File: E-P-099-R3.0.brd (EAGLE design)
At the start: 113.1 x 96.5 mm, 107 parts, among them J1 AVR_ISP, J2 1445055-3, Q1 BSS101, Q2 BSS101, Q3 BSS101, Q4 BSS101, Q5 BSS101, Q6 BSS101

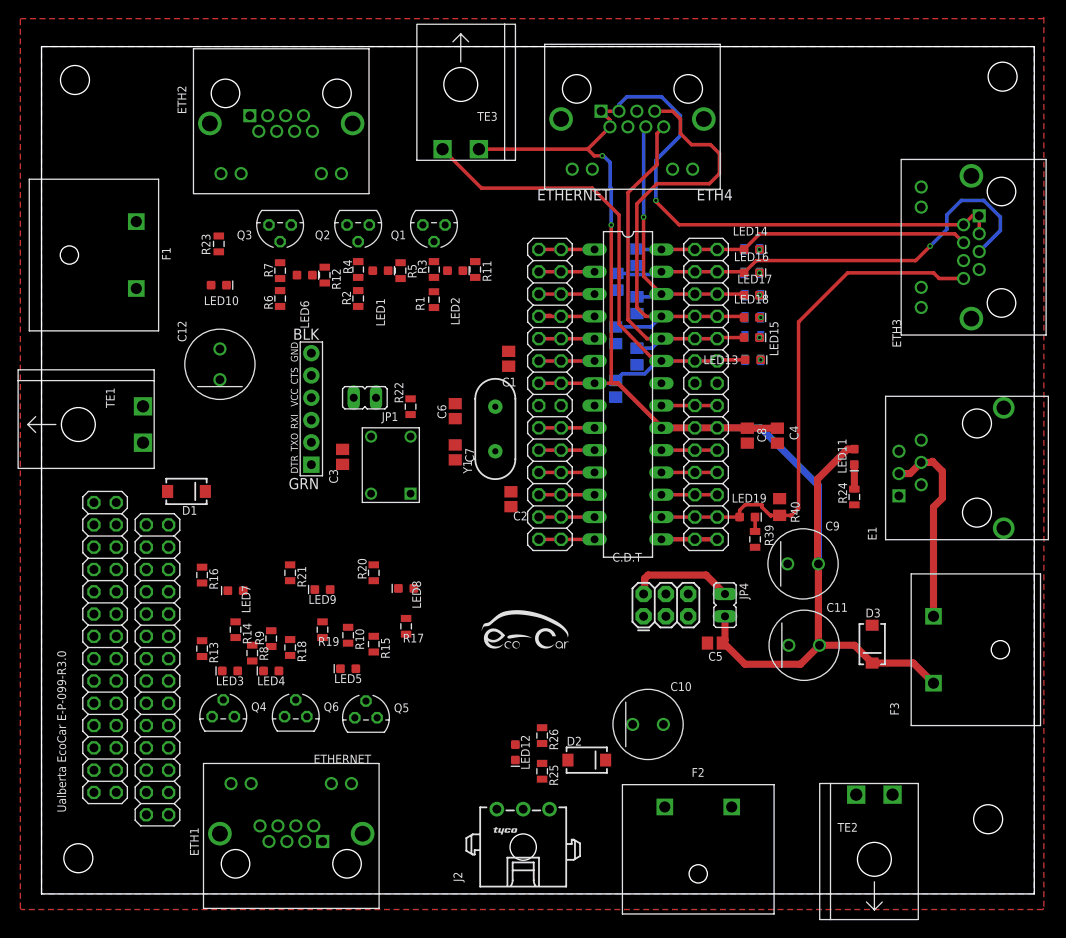
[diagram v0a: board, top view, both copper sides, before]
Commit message: update
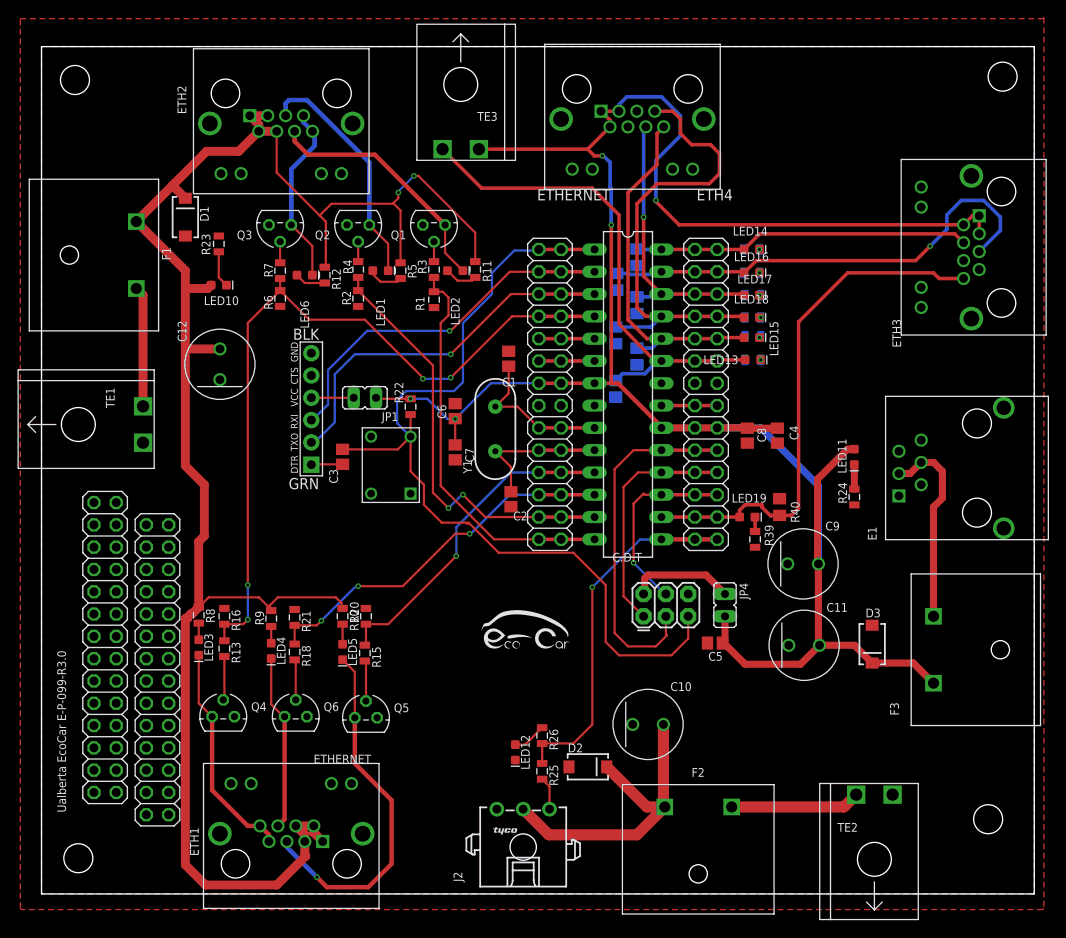
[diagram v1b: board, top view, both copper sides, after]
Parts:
- removed LED7, LED8, LED9: (no value), SparkFun-LED:LED-0603
- removed R14, R17, R19: 430, SparkFun-Passives:0805
- moved D1 31.2 mm to (16.4, 77.1), turned to 90 degrees
- moved R8 7.47 mm to (17.9, 31.8)
- moved R16 5.34 mm to (20.8, 31.6)
- moved R21 5.11 mm to (28.8, 31.5)
- moved R20 5.03 mm to (37.0, 31.6)
- moved LED3 4.45 mm to (17.9, 28.1), turned to 270 degrees
- moved R13 2.54 mm to (20.8, 27.9)
- moved LED4 2.29 mm to (26.2, 27.7), turned to 270 degrees
- moved R9 2.29 mm to (26.2, 31.4)
- moved R10 2.25 mm to (34.3, 31.6)
- moved LED5 2.01 mm to (34.3, 27.6), turned to 270 degrees
- moved R15 1.44 mm to (36.8, 27.4)
- moved D2 0.77 mm to (62.2, 14.5)
- moved R18 0.72 mm to (28.8, 27.6)
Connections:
- removed net N$41: LED8.C, R17.1
- removed net N$42: LED9.C, R19.1
- removed net N$44: LED7.C, R14.1
- net BRK_L_HIGH: no longer LED9.A
- net BRK_R_HIGH: no longer LED8.A
- net DRIVING_LIGHTS: no longer LED7.A
- net GND: no longer R14.2, R17.2, R19.2
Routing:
- net +12V: track 0.00 -> 205.7 mm, vias 0 -> 2
- net RESET: track 6.35 -> 103.4 mm
- net DRIVING_LIGHTS: track 7.81 -> 88.3 mm, vias 0 -> 4
- net BLINK_L: track 6.35 -> 48.9 mm, vias 0 -> 2
- net N$7: track 0.00 -> 41.1 mm, vias 0 -> 1
- net BLINK_R: track 6.79 -> 45.9 mm
- net SERVO_V: track 0.00 -> 36.6 mm
- net BRK_L_HIGH: track 6.35 -> 42.5 mm, vias 0 -> 3
- net TX: track 6.35 -> 42.5 mm, vias 0 -> 1
- net RX: track 6.53 -> 41.7 mm, vias 0 -> 1
- net SERVO: track 6.35 -> 41.1 mm, vias 0 -> 1
- net SCK: track 6.35 -> 40.6 mm
- net BRK_R_HIGH: track 6.35 -> 37.6 mm, vias 0 -> 1
- net N$21: track 0.00 -> 28.3 mm
- net N$22: track 0.00 -> 27.2 mm
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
